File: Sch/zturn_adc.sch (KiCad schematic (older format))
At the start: 1 part, among them IC1 CYUSB3014

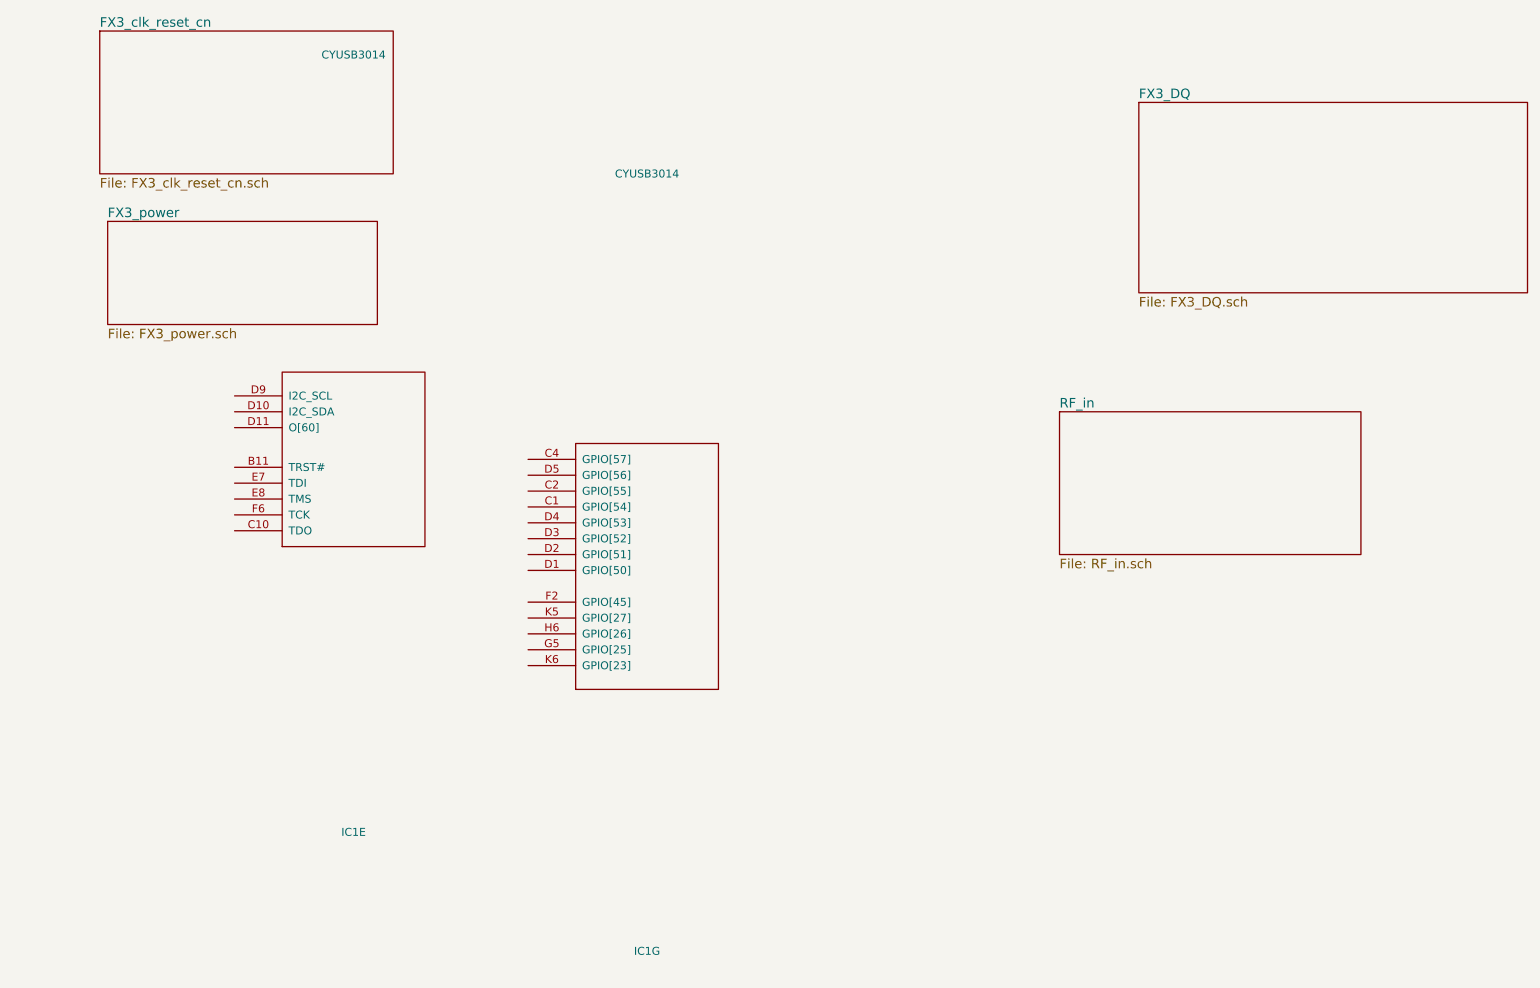
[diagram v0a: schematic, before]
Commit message: modify
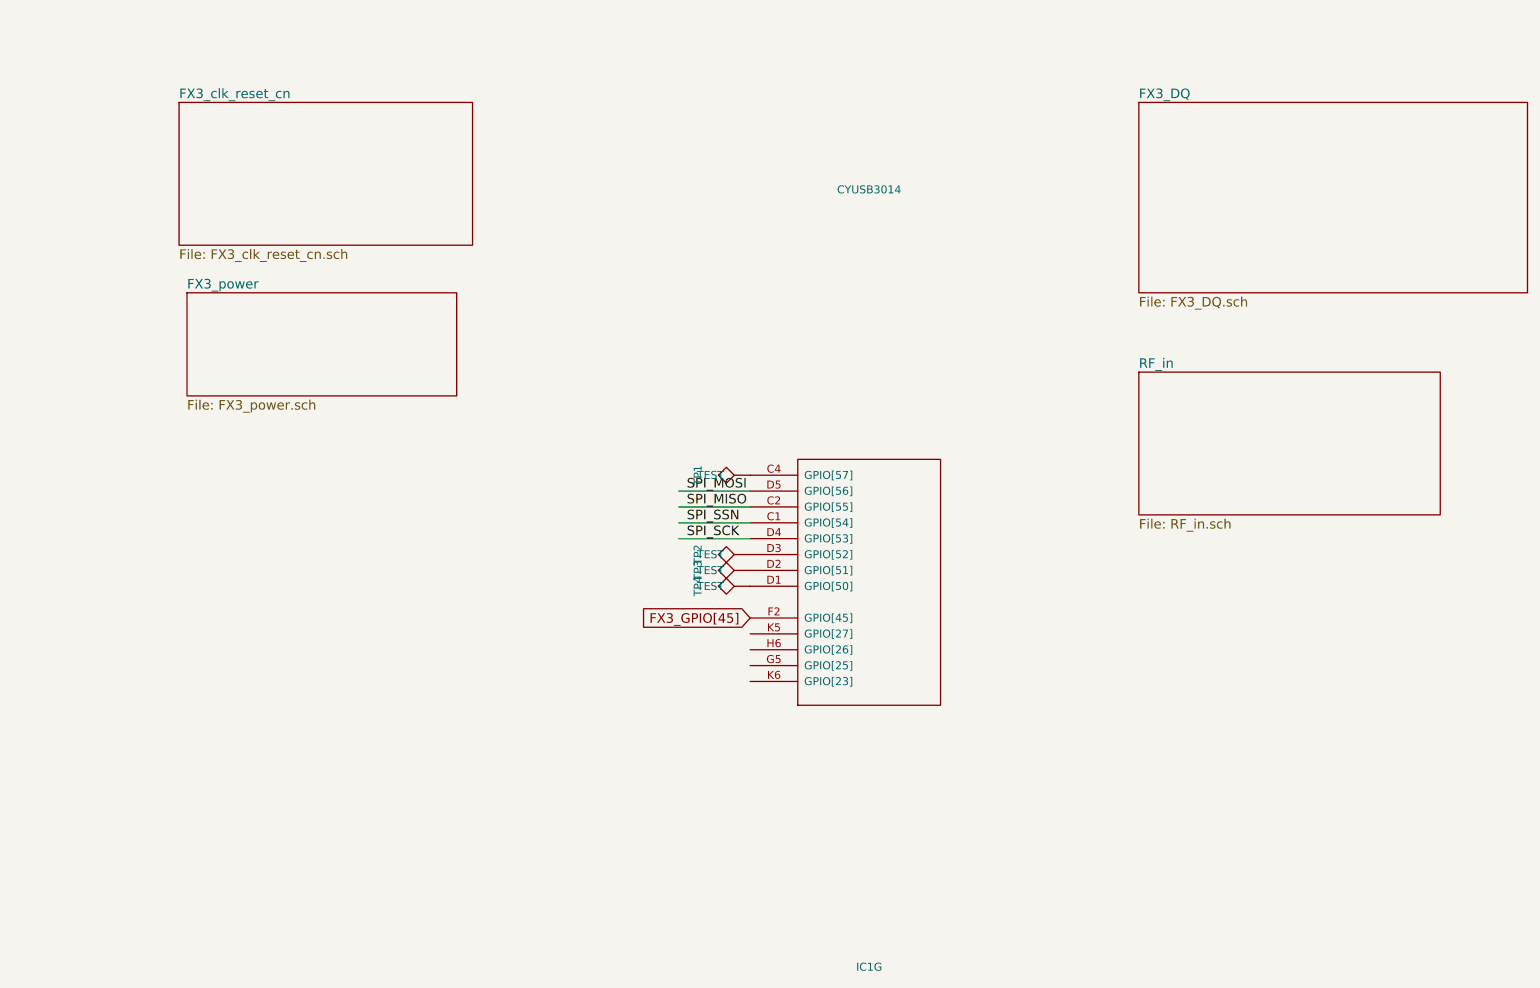
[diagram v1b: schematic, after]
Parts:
- removed unit 5 of IC1
- added TP1, TP2, TP3, TP4: TEST, symbol TEST
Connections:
- net labels added: FX3_GPIO[45], SPI_MISO, SPI_MOSI, SPI_SCK, SPI_SSN
- wire segments 0 -> 4
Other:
- moved on the sheet: IC1G
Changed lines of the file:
@@
 $EndDescr
 $Sheet
-S 1250 1200 1850 900
+S 1750 1650 1850 900
 U 589ADF9D
 F0 "FX3_clk_reset_cn" 60
@@
 $Comp
 L CYUSB3014 IC1
-U 5 1 58A0A752
-P 2850 3900
-F 0 "IC1" H 2850 1550 50  0000 C CNN
-F 1 "CYUSB3014" H 2850 6450 50  0000 C CNN
-F 2 "MODULE" H 2800 6200 50  0001 C CNN
-F 3 "DOCUMENTATION" H 2850 6350 50  0001 C CNN
-	5    2850 3900
-	1    0    0    -1
-$EndComp
-$Comp
-L CYUSB3014 IC1
 U 7 1 58A0A799
-P 4700 4650
-F 0 "IC1" H 4700 2300 50  0000 C CNN
-F 1 "CYUSB3014" H 4700 7200 50  0000 C CNN
-F 2 "MODULE" H 4650 6950 50  0001 C CNN
-F 3 "DOCUMENTATION" H 4700 7100 50  0001 C CNN
-	7    4700 4650
+P 6100 4750
+F 0 "IC1" H 6100 2400 50  0000 C CNN
+F 1 "CYUSB3014" H 6100 7300 50  0000 C CNN
+F 2 "MODULE" H 6050 7050 50  0001 C CNN
+F 3 "DOCUMENTATION" H 6100 7200 50  0001 C CNN
+	7    6100 4750
 	1    0    0    -1
 $EndComp
 $Sheet
-S 1300 2400 1700 650
+S 1800 2850 1700 650
 U 58A06B55
 F0 "FX3_power" 60
@@
 $EndSheet
 $Sheet
-S 7300 3600 1900 900
+S 7800 3350 1900 900
 U 58A1C0F3
 F0 "RF_in" 60
 F1 "RF_in.sch" 60
 $EndSheet
+Text Label 4950 4400 0    60   ~ 0
+SPI_SCK
+Text Label 4950 4300 0    60   ~ 0
+SPI_SSN
+Text Label 4950 4200 0    60   ~ 0
+SPI_MISO
+Text Label 4950 4100 0    60   ~ 0
+SPI_MOSI
+Wire Wire Line
+	5350 4400 4900 4400
+Wire Wire Line
+	5350 4300 4900 4300
+Wire Wire Line
+	5350 4200 4900 4200
+Wire Wire Line
+	5350 4100 4900 4100
+$Comp
+L TEST TP1
+U 1 1 58A3C918
+P 5350 4000
+F 0 "TP1" H 5350 4300 50  0000 C BNN
+F 1 "TEST" V 5350 4250 50  0000 C CNN
+F 2 "" H 5350 4000 50  0000 C CNN
+F 3 "" H 5350 4000 50  0000 C CNN
+	1    5350 4000
+	0    -1   -1   0
+$EndComp
+$Comp
+L TEST TP2
+U 1 1 58A3CCBA
+P 5350 4500
+F 0 "TP2" H 5350 4800 50  0000 C BNN
+F 1 "TEST" V 5350 4750 50  0000 C CNN
+F 2 "" H 5350 4500 50  0000 C CNN
+F 3 "" H 5350 4500 50  0000 C CNN
+	1    5350 4500
+	0    -1   -1   0
+$EndComp
+$Comp
+L TEST TP3
+U 1 1 58A3CCE7
+P 5350 4600
+F 0 "TP3" H 5350 4900 50  0000 C BNN
+F 1 "TEST" V 5350 4850 50  0000 C CNN
+F 2 "" H 5350 4600 50  0000 C CNN
+F 3 "" H 5350 4600 50  0000 C CNN
+	1    5350 4600
+	0    -1   -1   0
+$EndComp
+$Comp
+L TEST TP4
+U 1 1 58A3CFDC
+P 5350 4700
+F 0 "TP4" H 5350 5000 50  0000 C BNN
+F 1 "TEST" V 5350 4950 50  0000 C CNN
+F 2 "" H 5350 4700 50  0000 C CNN
+F 3 "" H 5350 4700 50  0000 C CNN
+	1    5350 4700
+	0    -1   -1   0
+$EndComp
+Text GLabel 5350 4900 0    60   Input ~ 0
+FX3_GPIO[45]
 $EndSCHEMATC

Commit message: update
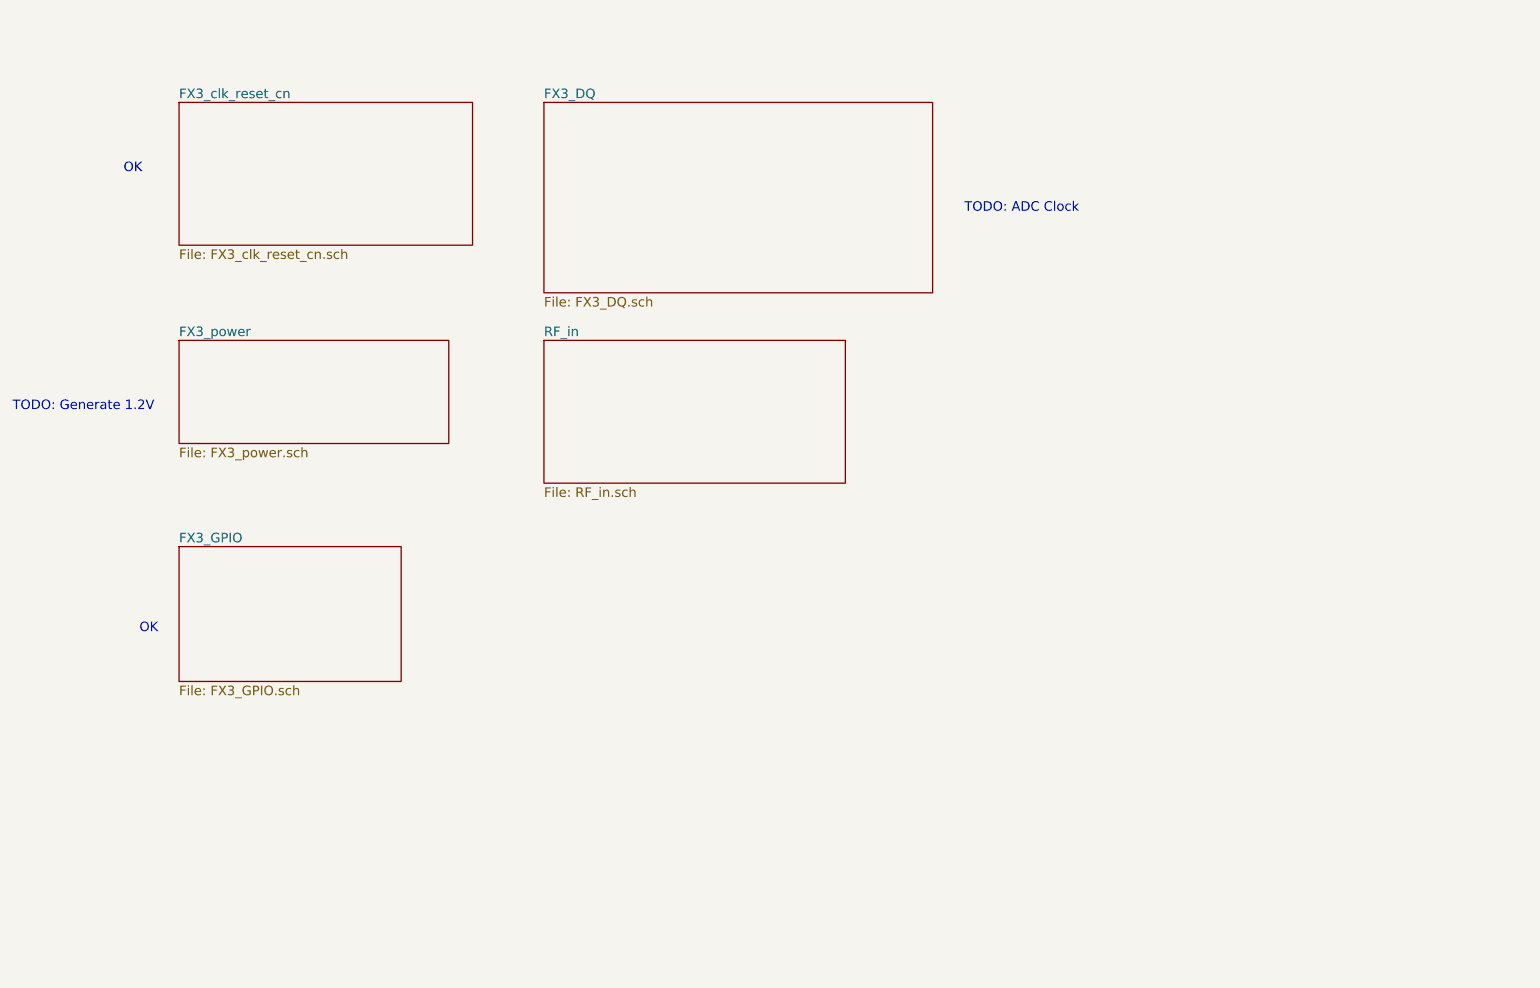
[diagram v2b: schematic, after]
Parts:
- removed IC1: CYUSB3014, MODULE, symbol CYUSB3014
- removed TP1, TP2, TP3, TP4: TEST, symbol TEST
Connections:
- net labels removed: FX3_GPIO[45], SPI_MISO, SPI_MOSI, SPI_SCK, SPI_SSN
- wire segments 4 -> 0
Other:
- note added: "OK"
- note added: "TODO: ADC Clock"
- note added: "TODO: Generate 1.2V"
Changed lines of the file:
@@
 $Descr A4 11693 8268
 encoding utf-8
-Sheet 1 5
+Sheet 1 6
 Title ""
 Date ""
@@
 F1 "FX3_clk_reset_cn.sch" 60
 $EndSheet
-$Comp
-L CYUSB3014 IC1
-U 7 1 58A0A799
-P 6100 4750
-F 0 "IC1" H 6100 2400 50  0000 C CNN
-F 1 "CYUSB3014" H 6100 7300 50  0000 C CNN
-F 2 "MODULE" H 6050 7050 50  0001 C CNN
-F 3 "DOCUMENTATION" H 6100 7200 50  0001 C CNN
-	7    6100 4750
-	1    0    0    -1
-$EndComp
 $Sheet
-S 1800 2850 1700 650
+S 1750 3150 1700 650
 U 58A06B55
 F0 "FX3_power" 60
@@
 $EndSheet
 $Sheet
-S 7800 1650 2450 1200
+S 4050 1650 2450 1200
 U 58A0A991
 F0 "FX3_DQ" 60
@@
 $EndSheet
 $Sheet
-S 7800 3350 1900 900
+S 4050 3150 1900 900
 U 58A1C0F3
 F0 "RF_in" 60
 F1 "RF_in.sch" 60
 $EndSheet
-Text Label 4950 4400 0    60   ~ 0
-SPI_SCK
-Text Label 4950 4300 0    60   ~ 0
-SPI_SSN
-Text Label 4950 4200 0    60   ~ 0
-SPI_MISO
-Text Label 4950 4100 0    60   ~ 0
-SPI_MOSI
-Wire Wire Line
-	5350 4400 4900 4400
-Wire Wire Line
-	5350 4300 4900 4300
-Wire Wire Line
-	5350 4200 4900 4200
-Wire Wire Line
-	5350 4100 4900 4100
-$Comp
-L TEST TP1
-U 1 1 58A3C918
-P 5350 4000
-F 0 "TP1" H 5350 4300 50  0000 C BNN
-F 1 "TEST" V 5350 4250 50  0000 C CNN
-F 2 "" H 5350 4000 50  0000 C CNN
-F 3 "" H 5350 4000 50  0000 C CNN
-	1    5350 4000
-	0    -1   -1   0
-$EndComp
-$Comp
-L TEST TP2
-U 1 1 58A3CCBA
-P 5350 4500
-F 0 "TP2" H 5350 4800 50  0000 C BNN
-F 1 "TEST" V 5350 4750 50  0000 C CNN
-F 2 "" H 5350 4500 50  0000 C CNN
-F 3 "" H 5350 4500 50  0000 C CNN
-	1    5350 4500
-	0    -1   -1   0
-$EndComp
-$Comp
-L TEST TP3
-U 1 1 58A3CCE7
-P 5350 4600
-F 0 "TP3" H 5350 4900 50  0000 C BNN
-F 1 "TEST" V 5350 4850 50  0000 C CNN
-F 2 "" H 5350 4600 50  0000 C CNN
-F 3 "" H 5350 4600 50  0000 C CNN
-	1    5350 4600
-	0    -1   -1   0
-$EndComp
-$Comp
-L TEST TP4
-U 1 1 58A3CFDC
-P 5350 4700
-F 0 "TP4" H 5350 5000 50  0000 C BNN
-F 1 "TEST" V 5350 4950 50  0000 C CNN
-F 2 "" H 5350 4700 50  0000 C CNN
-F 3 "" H 5350 4700 50  0000 C CNN
-	1    5350 4700
-	0    -1   -1   0
-$EndComp
-Text GLabel 5350 4900 0    60   Input ~ 0
-FX3_GPIO[45]
+$Sheet
+S 1750 4450 1400 850
+U 58A517F2
+F0 "FX3_GPIO" 60
+F1 "FX3_GPIO.sch" 60
+$EndSheet
+Text Notes 1500 5000 0    60   ~ 0
+OK
+Text Notes 1400 2100 0    60   ~ 0
+OK
+Text Notes 700  3600 0    60   ~ 0
+TODO: Generate 1.2V
+Text Notes 6700 2350 0    60   ~ 0
+TODO: ADC Clock
 $EndSCHEMATC
